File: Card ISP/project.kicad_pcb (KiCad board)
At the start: 2 copper layers, 51.5 x 22 mm, 15 parts, among them J1 ISP, U1 25/45/85, U2 168/328, X0 Card Edge, Y1 16Mhz

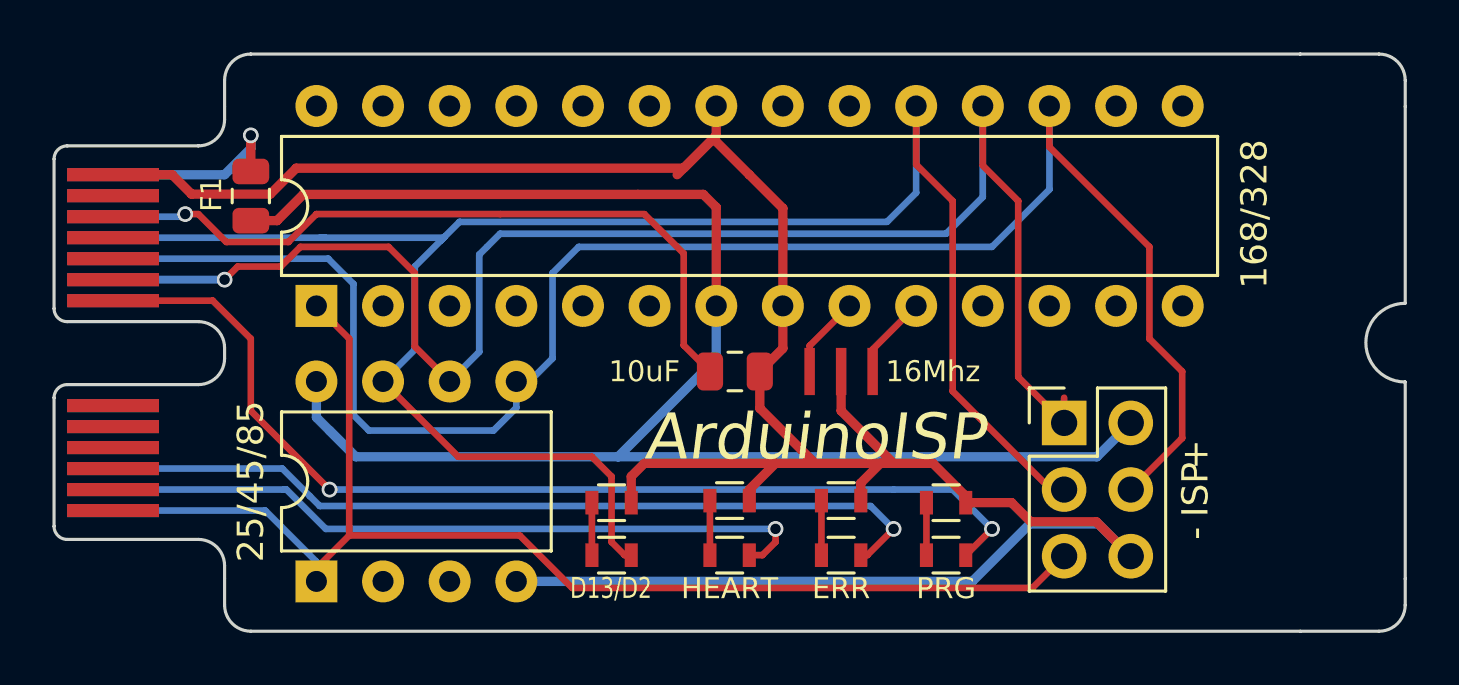
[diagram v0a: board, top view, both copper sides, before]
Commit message: Updates
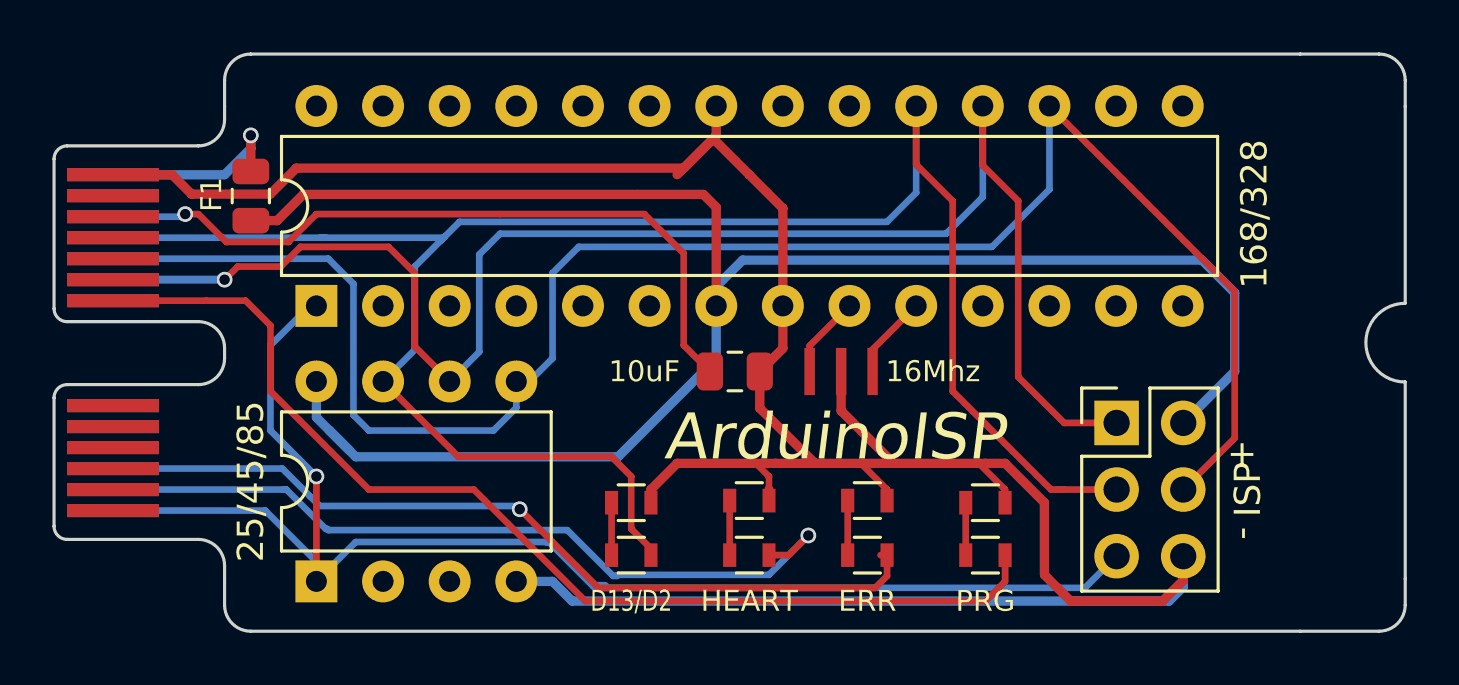
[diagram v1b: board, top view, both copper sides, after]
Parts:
- moved J1 2.00 mm to (40.5, -7.04)
- moved D3 1.50 mm to (35.5, -2.00)
- moved R4 1.50 mm to (35.5, -4.00)
- moved D2 1.00 mm to (31.0, -2.00)
- moved R3 1.00 mm to (31.0, -4.08)
- moved D1 0.75 mm to (26.5, -2.00)
- moved D4 0.75 mm to (22.0, -2.00)
- moved R1 0.75 mm to (22.0, -4.00)
- moved R2 0.75 mm to (26.5, -4.08)
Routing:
- net GND: track 96.6 -> 105.5 mm
- net +5V: track 64.0 -> 71.2 mm
- net /RST: track 49.4 -> 54.2 mm, vias 0 -> 1
- net /SCK: track 72.4 -> 75.2 mm
- net /LED_HB: track 27.6 -> 30.3 mm
- net /LED_PMODE: track 40.1 -> 41.5 mm, vias 2 -> 0
- net /MISO: track 60.3 -> 61.4 mm
- net /MOSI: track 68.3 -> 69.2 mm
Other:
- board text added: "- Remove card prior to programming base (dissables reset). - [File]->[Examples]->[ArduinoISP] - [Tools]->[Progammer]->[Arduino as ISP] - Insert card in X1 slot. - [Tools]->[Burn Bootloader] for Attiny to set clock speed."
- board text removed: "*Remove card prior to programming base (dissables reset)"
